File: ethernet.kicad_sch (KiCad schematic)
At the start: 1 part, among them U5 RTL8152B-VB-CG

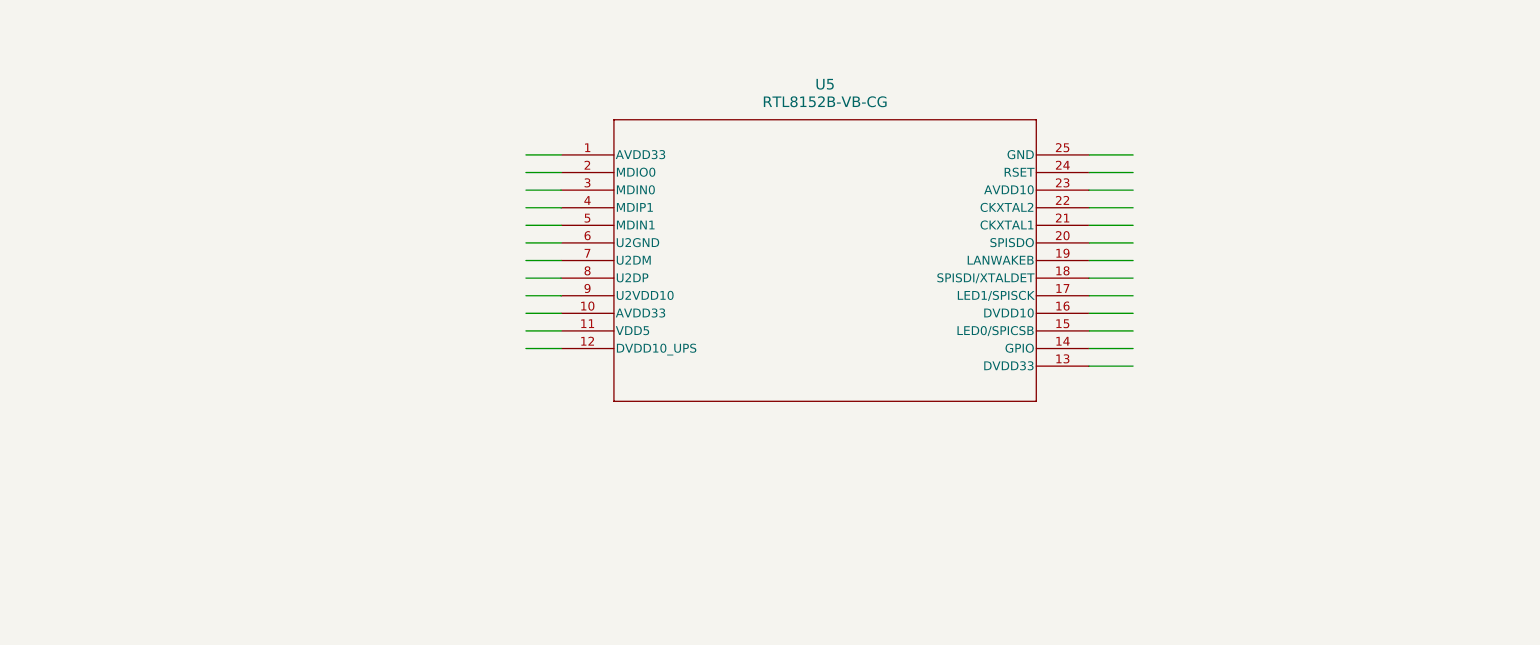
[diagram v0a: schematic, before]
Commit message: Add files via upload
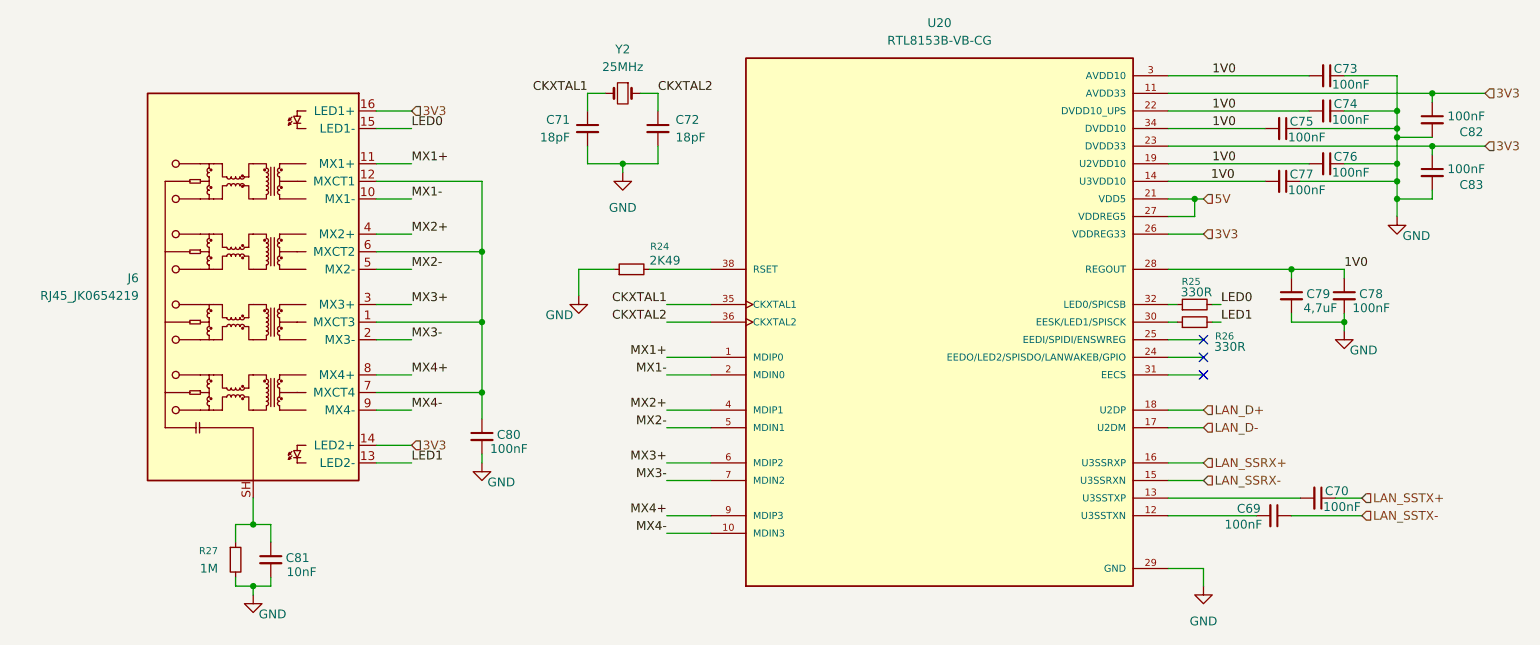
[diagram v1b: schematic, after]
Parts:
- removed U5: RTL8152B-VB-CG, RTL8152B-VB-CG_RTK, symbol RTL8152B-VB-CG:RTL8152B-VB-CG
- added C69, C70, C73, C74, C75, C76, C77, C78, C80, C82, C83: 100nF, symbol Device:C_Small
- added C71, C72: 18pF, symbol Device:C_Small
- added C79: 4,7uF, symbol Device:C_Small
- added C81: 10nF, symbol Device:C_Small
- added J6: RJ45_JK0654219, Connector_RJ:RJ45_Pulse_JK0654219NL_Horizontal, symbol Connector:RJ45_JK0654219
- added R24: 2K49, symbol Device:R_Small
- added R25, R26: 330R, symbol Device:R_Small
- added R27: 1M, symbol Device:R_Small
- added U20: RTL8153B-VB-CG, RTL8153B-VB-CG:QFN40P500X500X90-41N, symbol RTL8153B-VB-CG:RTL8153B-VB-CG
- added Y2: 25MHz, symbol Device:Crystal_Small
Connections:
- new net: R24.2, U20.38 (RSET)
- new net: C81.1, J6.SH, R27.1
- new net: R26.1, U20.30 (EESK/LED1/SPISCK)
- new net: C69.2, U20.12 (U3SSTXN)
- new net: C70.2, U20.13 (U3SSTXP)
- new net: R25.1, U20.32 (LED0/SPICSB)
- new net: C80.1, J6.1 (MXCT3), J6.12 (MXCT1), J6.6 (MXCT2), J6.7 (MXCT4)
- new net 5V: U20.21 (VDD5), U20.27 (VDDREG5)
- new net AVDD10: C73.2, C74.2, C75.2, C76.2, C77.2, C78.1, C79.1, U20.14 (U3VDD10), U20.19 (U2VDD10), U20.22 (DVDD10_UPS), U20.28 (REGOUT), U20.3 (AVDD10), U20.34 (DVDD10), U20.37 (AVDD10), U20.8 (AVDD10)
- new net AVDD33: C82.1, C83.1, J6.14 (LED2+), J6.16 (LED1+), U20.11 (AVDD33), U20.20 (AVDD33), U20.23 (DVDD33), U20.26 (VDDREG33), U20.33 (DVDD33), U20.39 (AVDD33), U20.40 (AVDD33)
- new net CKXTAL1: C71.1, U20.35 (CKXTAL1), Y2.2
- new net CKXTAL2: C72.1, U20.36 (CKXTAL2), Y2.1
- new net GND: C71.2, C72.2, C73.1, C74.1, C75.1, C76.1, C77.1, C78.2, C79.2, C80.2, C81.2, C82.2, C83.2, R24.1, R27.2, U20.29 (GND), U20.41 (GND)
- new net LAN_D+: U20.18 (U2DP)
- new net LAN_D-: U20.17 (U2DM)
- new net LAN_SSRX+: U20.16 (U3SSRXP)
- new net LAN_SSRX-: U20.15 (U3SSRXN)
- new net LAN_SSTX+: C70.1
- new net LAN_SSTX-: C69.1
- new net LED0: J6.15 (LED1-), R25.2
- new net LED1: J6.13 (LED2-), R26.2
- new net MX1+: J6.11 (MX1+), U20.1 (MDIP0)
- new net MX1-: J6.10 (MX1-), U20.2 (MDIN0)
- new net MX2+: J6.4 (MX2+), U20.4 (MDIP1)
- new net MX2-: J6.5 (MX2-), U20.5 (MDIN1)
- new net MX3+: J6.3 (MX3+), U20.6 (MDIP2)
- new net MX3-: J6.2 (MX3-), U20.7 (MDIN2)
- new net MX4+: J6.8 (MX4+), U20.9 (MDIP3)
- new net MX4-: J6.9 (MX4-), U20.10 (MDIN3)
- no-connect marks 0 -> 3
